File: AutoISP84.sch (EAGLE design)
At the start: 4 parts, among them J1 MCU, J2 BOARD, U1 ATTINY84-20PU, U2 ATTINY84-20PU

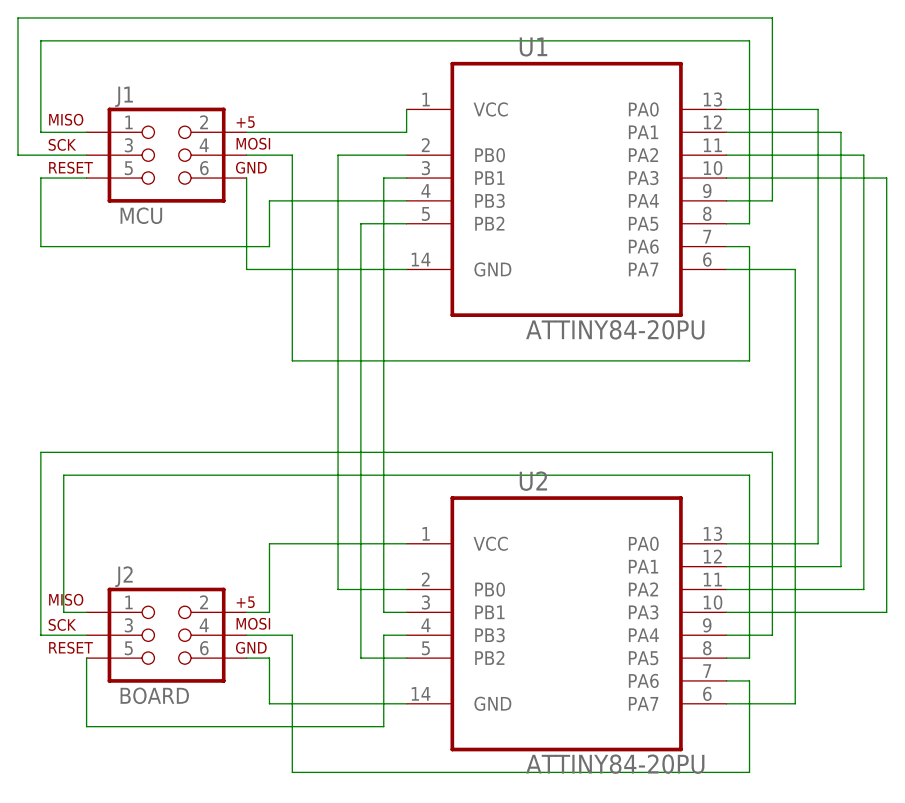
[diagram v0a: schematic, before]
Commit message: Revise boards for better labelling and sane orientation, add AutoISP328
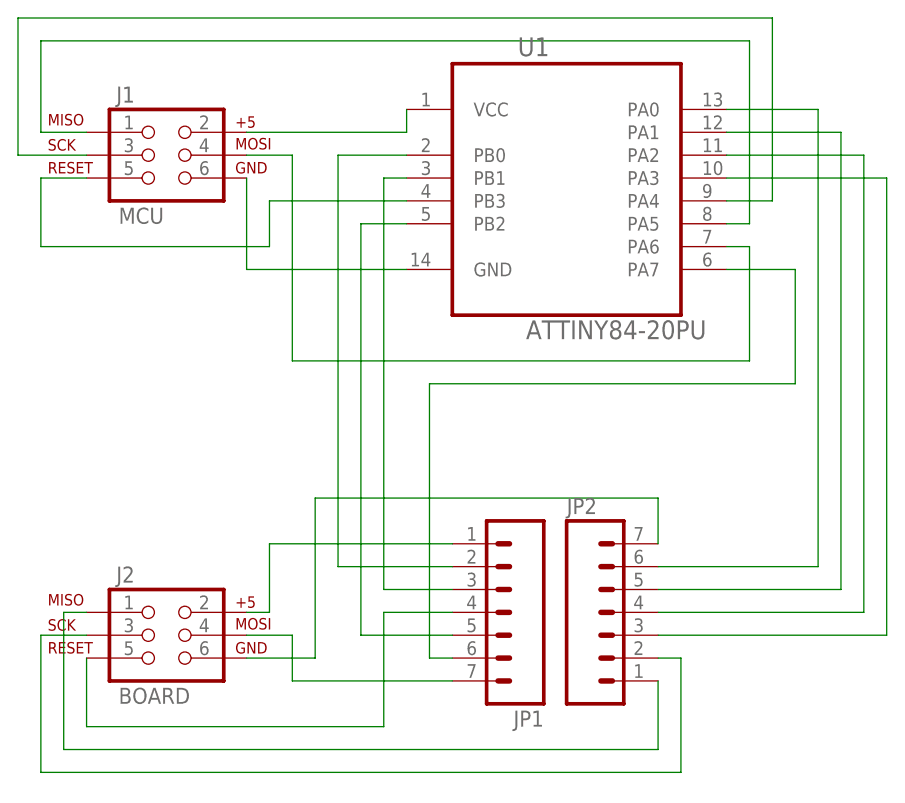
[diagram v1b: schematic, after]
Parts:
- removed U2: ATTINY84-20PU, Atmel_By_element14_Batch_1-00:ATTINY84-20PU
- added JP1, JP2: (no value), SparkFun-Connectors:M07POGOPINS_HOLES_ONLY
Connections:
- removed net N$11: J2.1, U2.PA5
- removed net N$13: J2.3, U2.PA4
- removed net N$9: J2.4, U2.PA6
- new net N$19: J2.4, JP1.7
- new net N$22: J2.1, JP2.1
- new net N$23: J2.3, JP2.2
- net N$12: now also JP2.6; no longer U2.PA0
- net N$14: now also JP1.5; no longer U2.PB2
- net N$15: now also JP1.3; no longer U2.PB1
- net N$16: now also JP1.2; no longer U2.PB0
- net N$17: now also JP1.6; no longer U2.PA7
- net N$18: now also JP2.5; no longer U2.PA1
- net N$2: now also JP1.1; no longer U2.VCC
- net N$20: now also JP2.4; no longer U2.PA2
- net N$21: now also JP2.3; no longer U2.PA3
- net N$3: now also JP2.7; no longer U2.GND
- net N$7: now also JP1.4; no longer U2.PB3

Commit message: AutoISP85 1.3 (Fix flipped pin header) Add BOM
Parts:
- JP1, JP2: device SparkFun-Connectors:M07POGOPINS_HOLES_ONLY -> SparkFun-Connectors:M07
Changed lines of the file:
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@@
 <part name="J2" library="SparkFun-Connectors" deviceset="AVR_SPI_PRG_6" device="PTH" value="BOARD"/>
 <part name="U1" library="Atmel_By_element14_Batch_1-00" deviceset="ATTINY84-20PU" device=""/>
-<part name="JP1" library="SparkFun-Connectors" deviceset="M07" device="POGOPINS_HOLES_ONLY"/>
-<part name="JP2" library="SparkFun-Connectors" deviceset="M07" device="POGOPINS_HOLES_ONLY"/>
+<part name="JP1" library="SparkFun-Connectors" deviceset="M07" device=""/>
+<part name="JP2" library="SparkFun-Connectors" deviceset="M07" device=""/>
 </parts>
 <sheets>
